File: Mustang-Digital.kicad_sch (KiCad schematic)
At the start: 0 parts

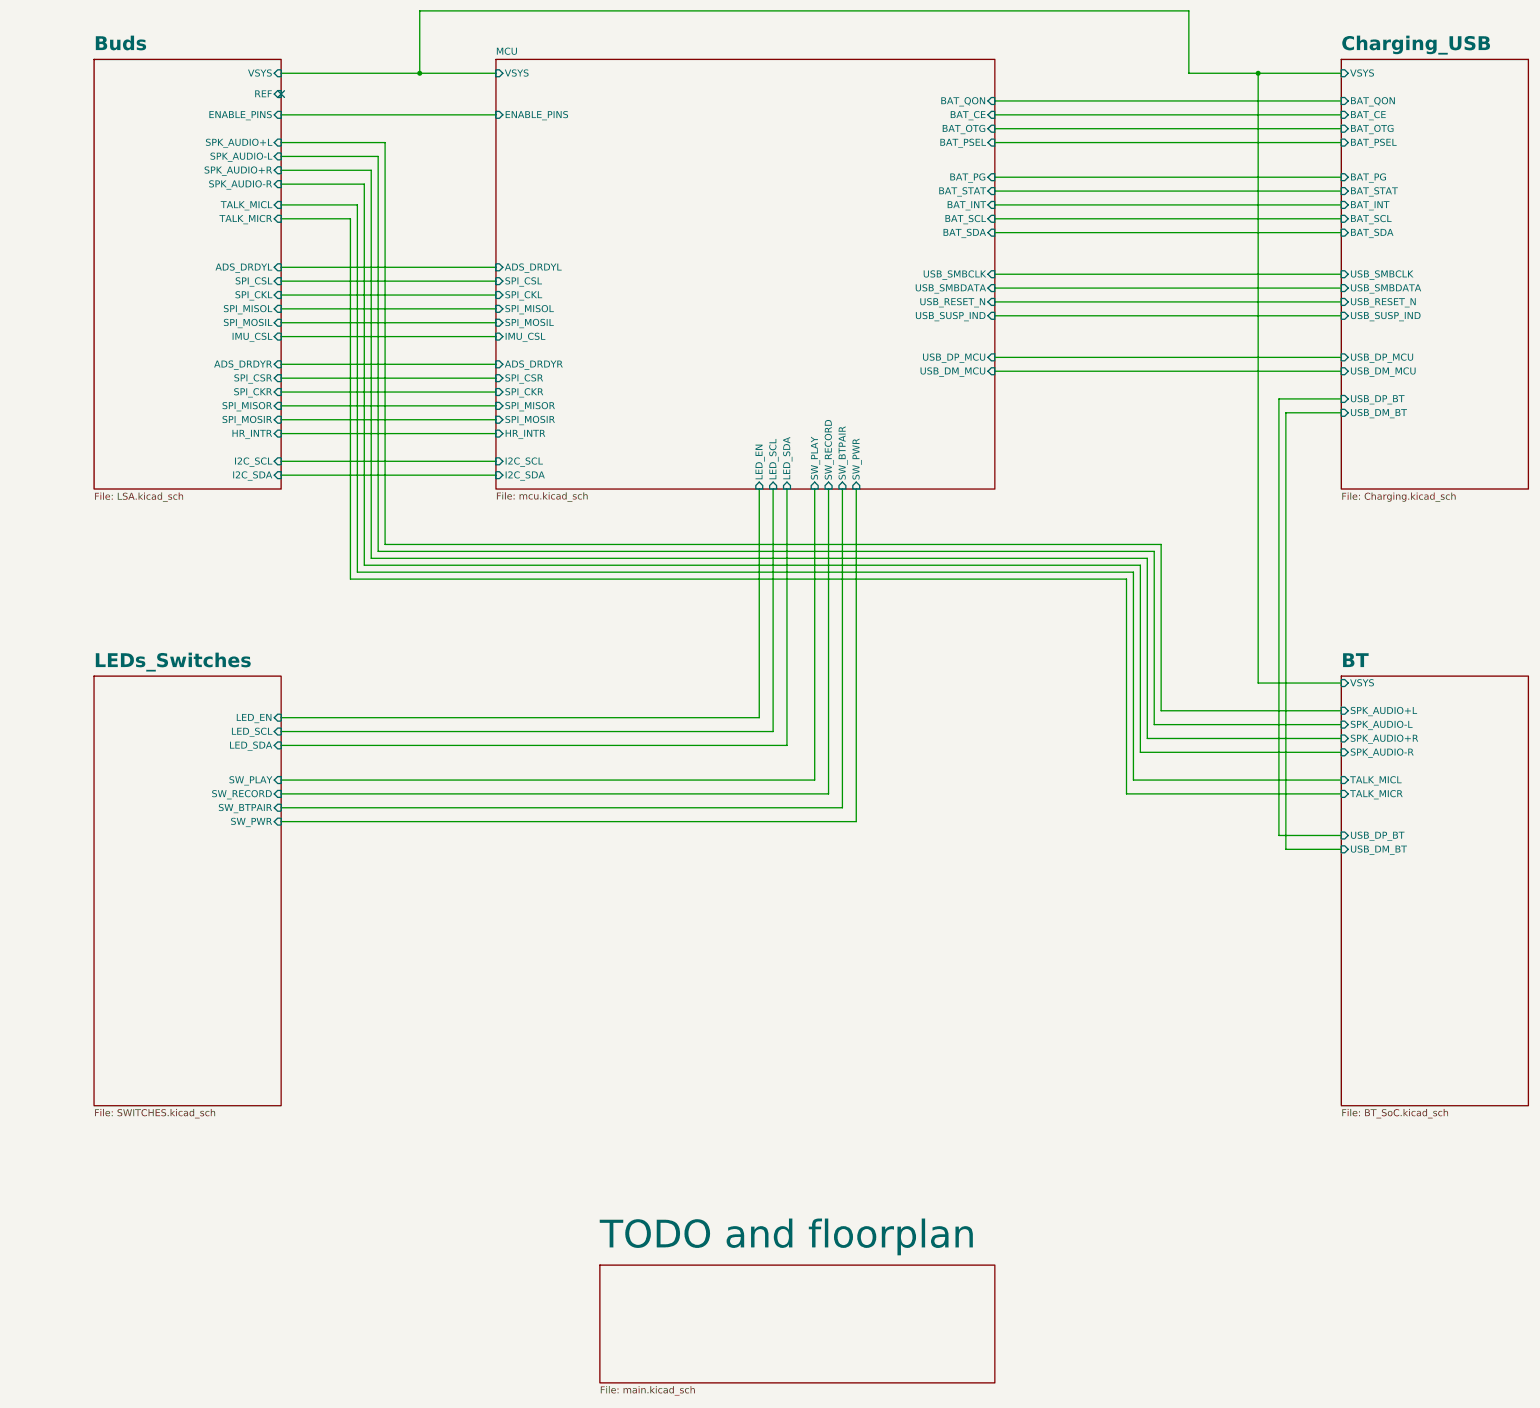
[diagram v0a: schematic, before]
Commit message: wip
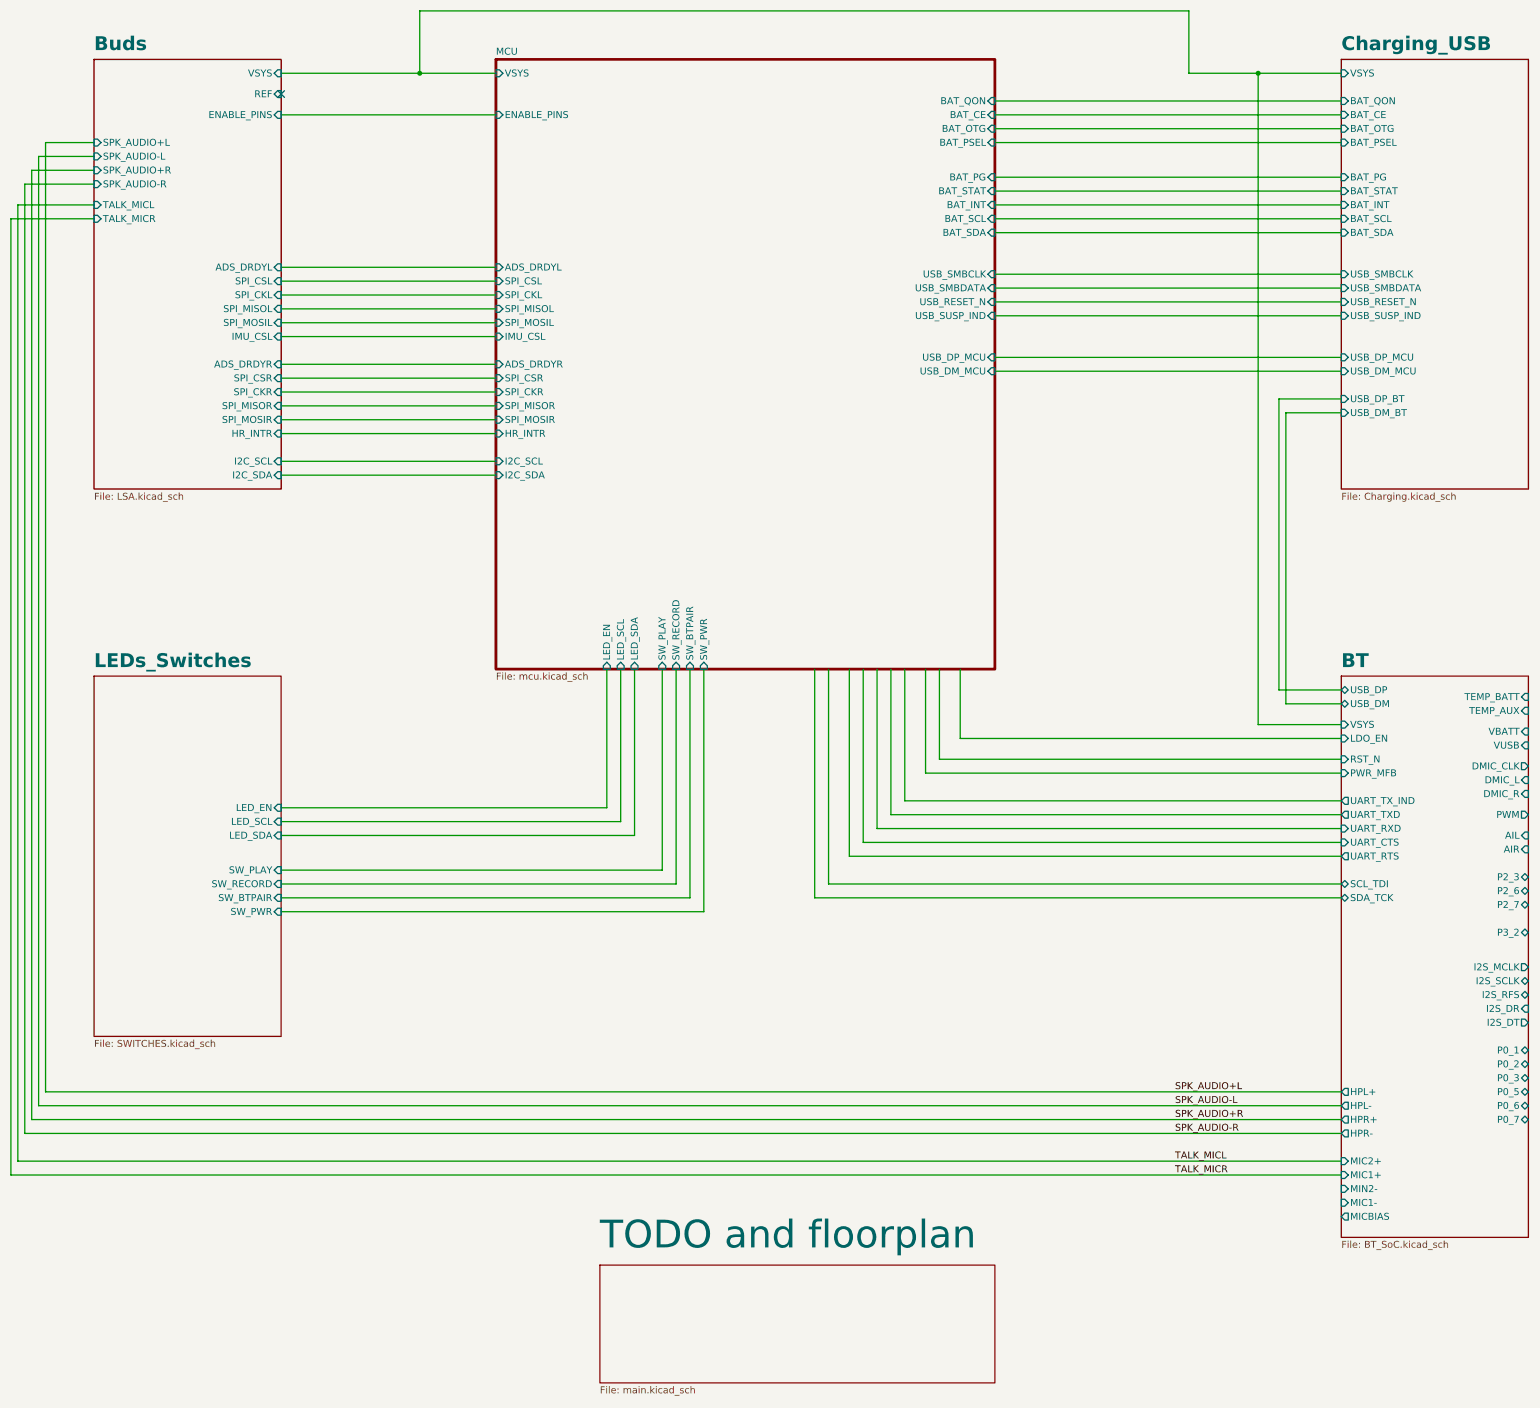
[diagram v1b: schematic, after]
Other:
- sheet BT ports: added AIL, AIR, DMIC_CLK, DMIC_L, DMIC_R, HPL+, HPL-, HPR+, HPR-, I2S_DR, I2S_DT, I2S_MCLK, I2S_RFS, I2S_SCLK, LDO_EN, MIC1+, MIC1-, MIC2+, MICBIAS, MIN2-, P0_1, P0_2, P0_3, P0_5, P0_6, P0_7, P2_3, P2_6, P2_7, P3_2, PWM, PWR_MFB, RST_N, SCL_TDI, SDA_TCK, TEMP_AUX, TEMP_BATT, UART_CTS, UART_RTS, UART_RXD, UART_TXD, UART_TX_IND, USB_DM, USB_DP, VBATT, VUSB; removed SPK_AUDIO+L, SPK_AUDIO+R, SPK_AUDIO-L, SPK_AUDIO-R, TALK_MICL, TALK_MICR, USB_DM_BT, USB_DP_BT
